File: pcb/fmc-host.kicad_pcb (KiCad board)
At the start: 6 copper layers, 76.5 x 339.8 mm, 310 parts, among them J1 6-1634010-0, J10 BM08B-SURS-TF, J2 6-1634010-0, J3 6-1634010-0, J4 6-1634010-0, J5 6-1634010-0, J6 FTSH-105-01-F-D-RA-K, J7 12226-8250-00FR, J8 FMC_SINGLE_WIDTH_MODULE, J9 ASP-134488-01, Q1 SI1012R, Q2 SI1012R, U1 SN74LVC2G34DCKR, U10 DS90UB934-Q1, U11 DS91M040, U12 AD5766BCPZ-RL7, U13 MCP47FEB02A0-E/ST, U14 LM4132AMF-2.5/NOPB, U15 AD7616BSTZ, U16 AD5142BRUZ10, U17 LTM4622A, U18 D3V3XA4B10LP, U19 TPS7A49, U2 SN65LVDS9638DGN, U20 TPS7A49, U21 TPS7A30, U22 24AA64-I/ST, U23 LTM8049IY#PBF, U24 TPS62061DSGT, U25 D3V3XA4B10LP, U26 D3V3XA4B10LP, U3 FIN1032MTCX, U4 ADCMP600, U5 ADCMP600, U6 DG1412E, U7 DG1412E, U8 DG1412E, U9 DS90UB934-Q1, X2 OE-LOGO_7X5

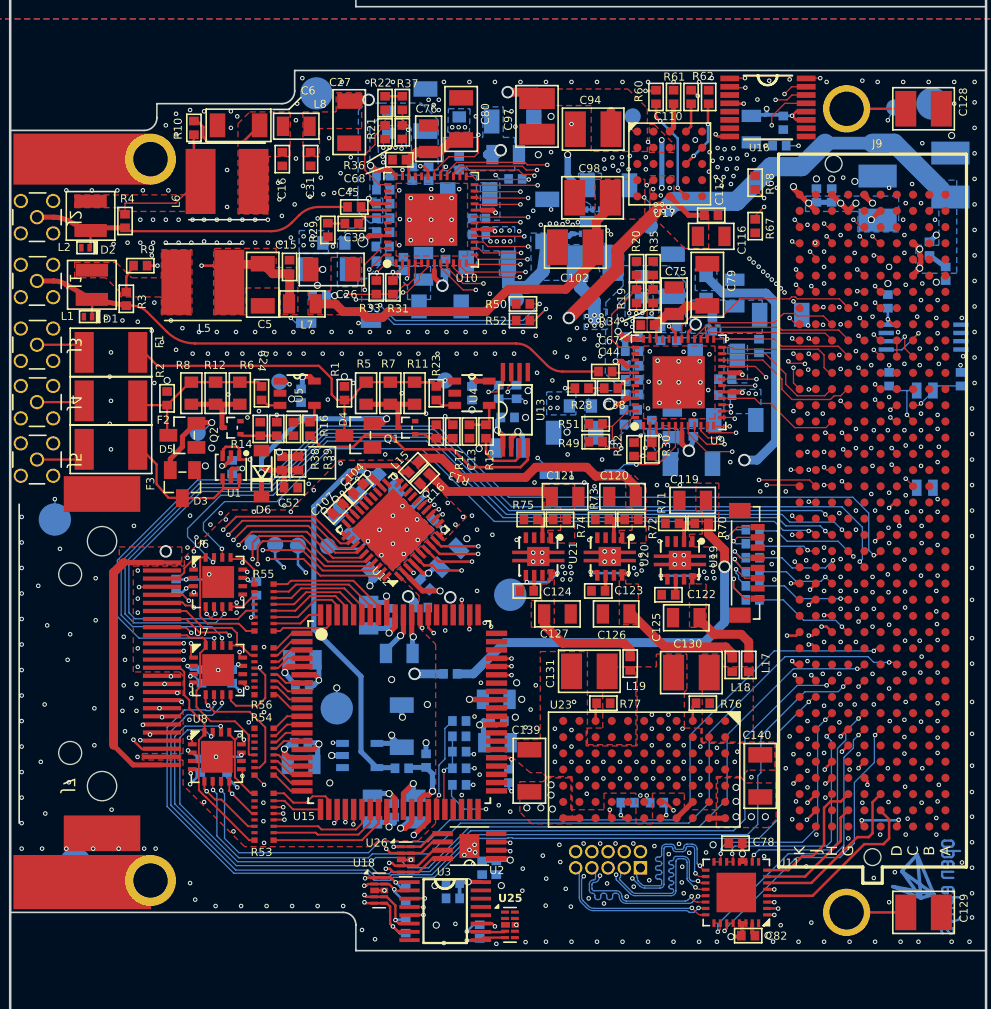
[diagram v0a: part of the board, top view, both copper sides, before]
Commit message: Address EDADOCs EQs for rev. g
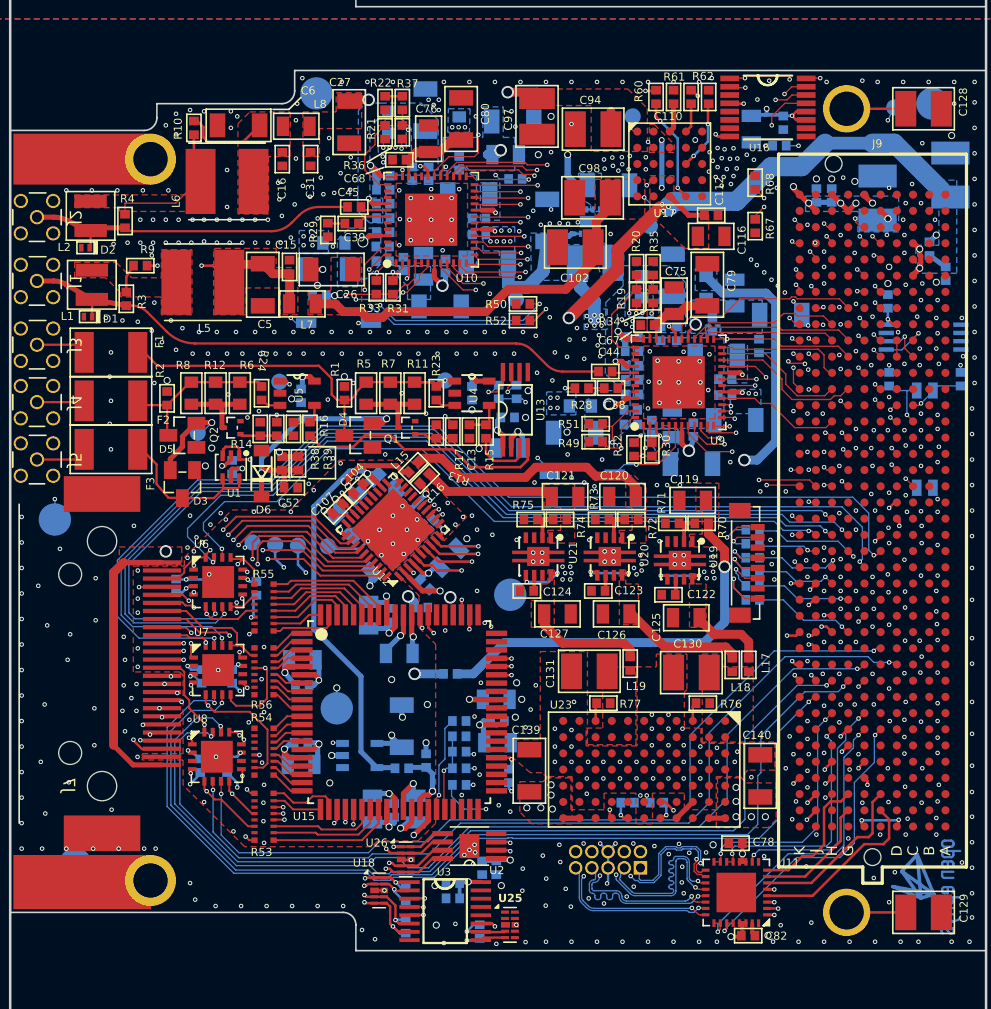
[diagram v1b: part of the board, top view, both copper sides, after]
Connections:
- J6 pad 05: unconnected-(J6-5-Pad05) -> GND
- J6 pad 06: unconnected-(J6-6-Pad06) -> GND
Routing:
- net /MLVDS_CLK_3_P: track 13.6 -> 10.7 mm
- net Net-(D4-COMM): track 33.2 -> 31.6 mm
- net /LVDS_DOUT1_N: track 34.4 -> 32.9 mm
- net /AIO_4: track 16.5 -> 15.3 mm, vias 0 -> 2
- net /AIO_11: track 13.7 -> 14.9 mm, vias 0 -> 2
- net /MLVDS_CLK_3_N: track 13.9 -> 12.7 mm
- net +3V3: track 101.7 -> 100.6 mm
- net GND: track 24.3 -> 25.3 mm, vias 729 -> 723
- net AGND: track 55.9 -> 55.1 mm, vias 55 -> 57
- net Net-(U15-REFSEL): track 8.24 -> 7.44 mm
- net Net-(U9-IDX): track 6.23 -> 5.45 mm
- net +12V: track 123.2 -> 122.6 mm, vias 16 -> 11
- net /AIO_0: track 18.0 -> 18.5 mm, vias 0 -> 2
- net /+5V_AN: track 29.5 -> 28.9 mm
- net /AIO_6: track 16.9 -> 17.4 mm
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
